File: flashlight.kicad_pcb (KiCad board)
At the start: 2 copper layers, 45 x 120 mm, 23 parts, among them J1 USB_B_Micro, J2 Conn_01x03_Pin, Q2 HSS2333, SW1 SW_DIP_x01, U1 XB4908A, U2 MT3608, U3 TP4057, U4 R6BHC-A05_LED-19-223

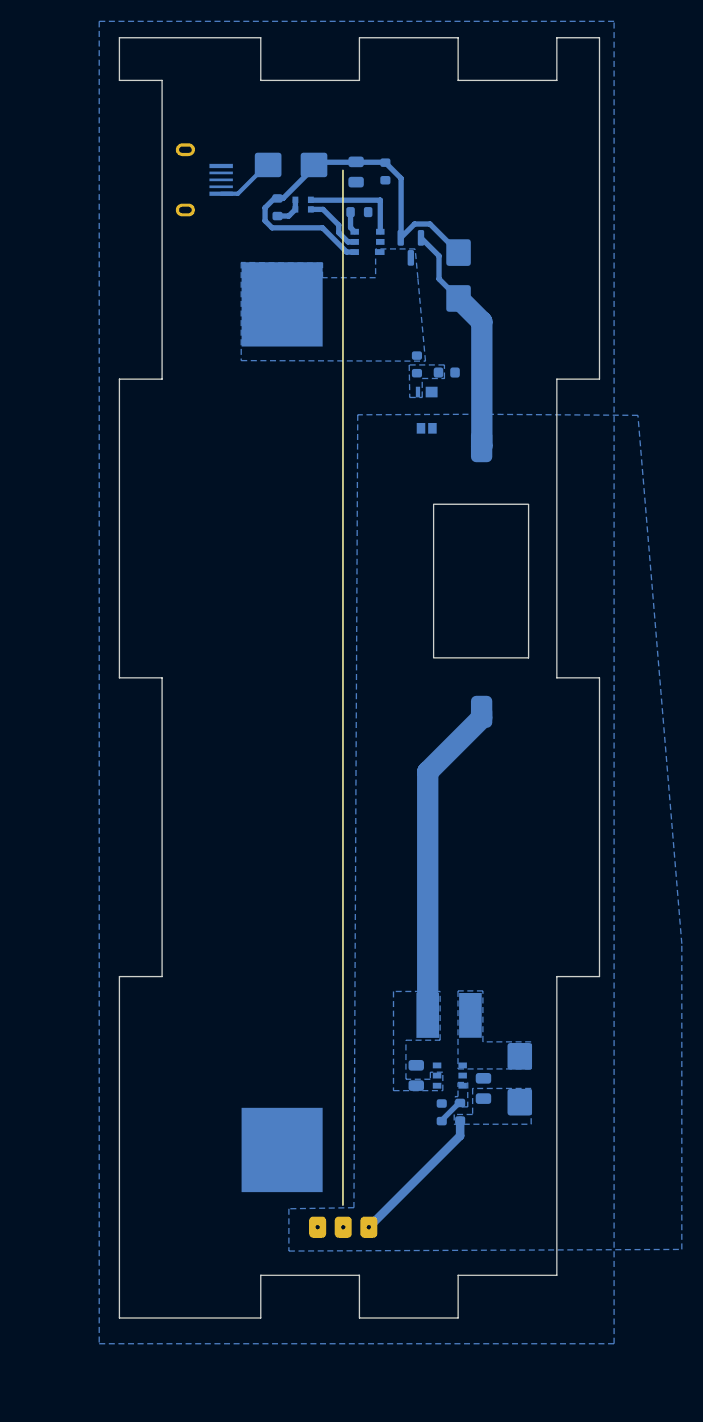
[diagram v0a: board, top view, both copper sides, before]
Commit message: v2.7 boxes
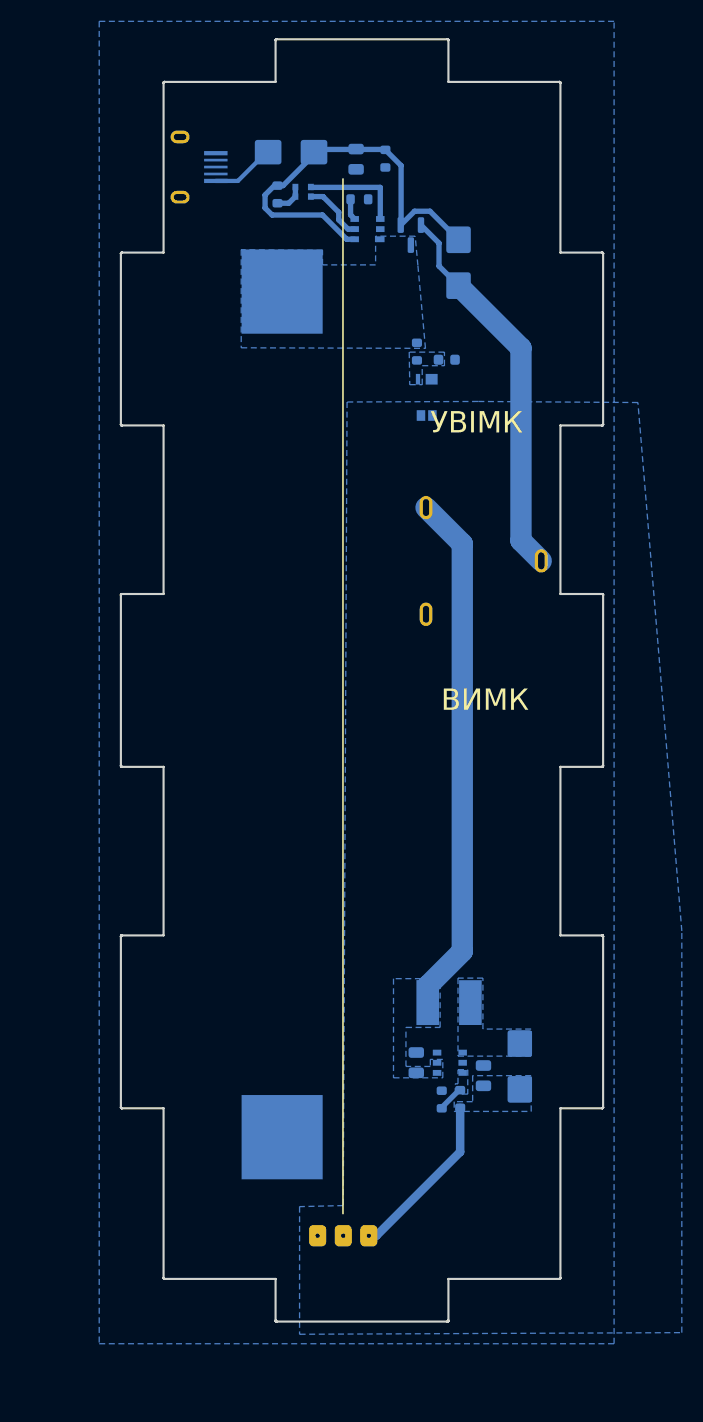
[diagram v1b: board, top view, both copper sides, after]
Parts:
- removed SW1: SW_DIP_x01, FlashlightLib:KCD11-2P
- added U5: SS12J01_071, JLCPCB-SS12J01:SW-TH_SHOU-HAN_SS12J01, F.Cu at (109.2, 84.6)
- moved J1 1.30 mm to (82.5, 47.7)
- moved C3 1.20 mm to (102.9, 131.6)
- moved C4 1.20 mm to (109.2, 132.9)
- moved R6 1.20 mm to (105.3, 135.1)
- moved U2 1.20 mm to (106.0, 131.7)
- moved BT1 1.20 mm to (90.3, 99.0)
- moved C1 1.20 mm to (97.2, 47.0)
- moved C2 1.20 mm to (105.7, 65.8)
- moved Q2 1.20 mm to (102.4, 54.1)
- moved R1 1.20 mm to (97.5, 50.7)
- moved R2 1.20 mm to (89.9, 50.3)
- moved R3 1.20 mm to (102.9, 65.0)
- moved U1 1.20 mm to (103.1, 67.6)
- moved U4 1.20 mm to (93.0, 49.5)
- moved D1 1.20 mm to (91.1, 46.3)
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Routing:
- net Net-(U2-EN): track 30.5 -> 49.1 mm
- net Net-(D4-K): track 21.9 -> 36.2 mm
- net VOUT: track 13.5 -> 16.0 mm
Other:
- board size 45 x 120 mm -> 45.2 x 120.2 mm
- board text added: "DO NOT PRINT ON F LAYER!"
- board text added: "V2.7"
- board text added: "ВИМК"
- board text added: "УВІМК"
- board text removed: "V2.6"

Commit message: V3.0 21700 3x8 leds
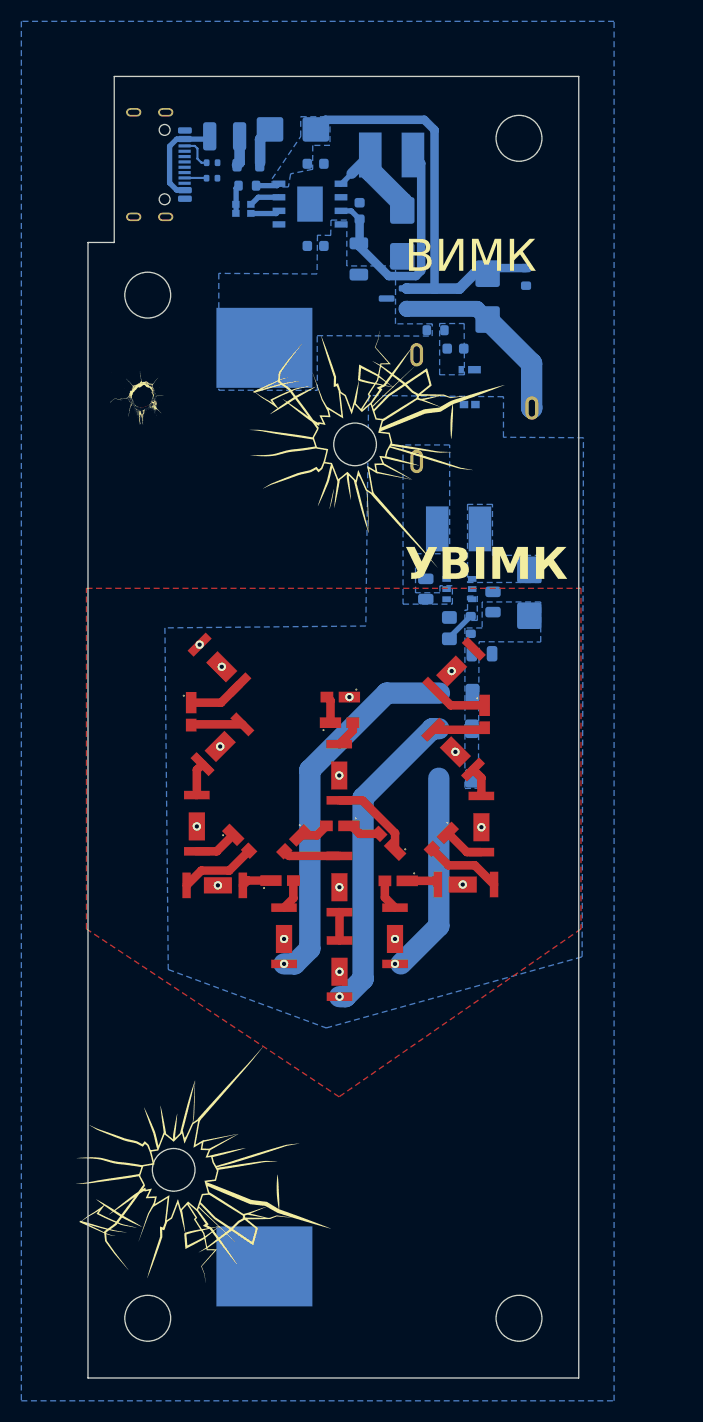
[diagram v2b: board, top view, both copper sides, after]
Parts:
- removed J1: USB_B_Micro, FlashlightLib:USB-1101IPX6-02
- removed J2: Conn_01x03_Pin, FlashlightLib:LED_Strip
- added C4: 22uF/35V, Capacitor_SMD:C_0805_2012Metric, B.Cu at (109.0, 93.3)
- added C5: 10uF/10V, Capacitor_SMD:C_0603_1608Metric, B.Cu at (97.6, 51.8)
- added C6: 10uF/10V, Capacitor_SMD:C_0603_1608Metric, B.Cu at (93.4, 55.1)
- added D10: LED, footprint:LED-SMD_L3.0-W1.4-RD_WHITE, F.Cu at (81.8, 98.9)
- added D11: LED_Pad, footprint:LED-SMD_3P-L5.7-W3.0-RD, F.Cu at (84.4, 94.3)
- added D12: LED_Pad, footprint:LED-SMD_3P-L5.7-W3.0-RD, F.Cu at (95.7, 122.8)
- added D13: LED_Pad, footprint:LED-SMD_3P-L5.7-W3.0-RD, F.Cu at (95.7, 114.9)
- added D14: LED, footprint:LED-SMD_L3.0-W1.4-RD_WHITE, F.Cu at (91.2, 111.1)
- added D15: LED, footprint:LED-SMD_L3.0-W1.4-RD_WHITE, F.Cu at (95.5, 109.4)
- added D16: LED, footprint:LED-SMD_L3.0-W1.4-RD_WHITE, F.Cu at (100.1, 110.9)
- added D17: LED_Pad, footprint:LED-SMD_3P-L5.7-W3.0-RD, F.Cu at (95.7, 104.4)
- added D18: LED, footprint:LED-SMD_L3.0-W1.4-RD_WHITE, F.Cu at (95.9, 99.8)
- added D19: LED, footprint:LED-SMD_L3.0-W1.4-RD_WHITE, F.Cu at (95.6, 97.4)
- added D2: D_Schottky, Diode_SMD:D_SMB, B.Cu at (101.6, 53.9)
- added D20: LED_Pad, footprint:LED-SMD_3P-L5.7-W3.0-RD, F.Cu at (106.4, 94.7)
- added D21: LED, footprint:LED-SMD_L3.0-W1.4-RD_WHITE, F.Cu at (109.3, 99.2)
- added D22: LED_Pad, footprint:LED-SMD_3P-L5.7-W3.0-RD, F.Cu at (106.3, 102.3)
- added D23: LED_Pad, footprint:LED-SMD_3P-L5.7-W3.0-RD, F.Cu at (109.0, 109.3)
- added D24: LED, footprint:LED-SMD_L3.0-W1.4-RD_WHITE, F.Cu at (105.1, 110.8)
- added D25: LED_Pad, footprint:LED-SMD_3P-L5.7-W3.0-RD, F.Cu at (107.5, 114.9)
- added D26: LED, footprint:LED-SMD_L3.0-W1.4-RD_WHITE, F.Cu at (101.0, 114.6)
- added D27: LED_Pad, footprint:LED-SMD_3P-L5.7-W3.0-RD, F.Cu at (100.9, 119.7)
- added D28: LED_Pad, footprint:LED-SMD_3P-L5.7-W3.0-RD, F.Cu at (90.5, 119.7)
- added D3: LED, footprint:LED-SMD_L3.0-W1.4-RD_WHITE, F.Cu at (90.3, 114.6)
- added D6: LED_Pad, footprint:LED-SMD_3P-L5.7-W3.0-RD, F.Cu at (84.0, 115.0)
- added D7: LED, footprint:LED-SMD_L3.0-W1.4-RD_WHITE, F.Cu at (86.5, 111.0)
- added D8: LED_Pad, footprint:LED-SMD_3P-L5.7-W3.0-RD, F.Cu at (82.3, 109.2)
- added D9: LED_Pad, footprint:LED-SMD_3P-L5.7-W3.0-RD, F.Cu at (84.7, 101.8)
- added F2: BSMD1210-150-6V, Fuse:Fuse_1210_3225Metric, B.Cu at (84.9, 44.8)
- added FB1: FerriteBead, Inductor_SMD:L_0805_2012Metric, B.Cu at (87.1, 47.5)
- added G***: LOGO, LOGO, F.Cu at (76.7, 69.3)
- added G***: LOGO, LOGO, F.Cu at (99.0, 74.0)
- added H1: MountingHole, FlashlightLib:M4-insert, F.Cu at (77.7, 59.7)
- added H2: MountingHole, FlashlightLib:M4-insert, F.Cu at (112.5, 45.0)
- added H3: MountingHole, FlashlightLib:M4-insert, F.Cu at (77.7, 155.6)
- added H4: MountingHole, FlashlightLib:M4-insert, F.Cu at (112.5, 155.6)
- added J11: USB_C_Receptacle_USB2.0_16P, footprint:USB-SMD_GT-USB-7070A01, B.Cu at (78.8, 47.5)
- added L2: 10uH, FlashlightLib:L_5.0x5.0, B.Cu at (100.6, 46.6)
- added R20: 5.1k, Resistor_SMD:R_0402_1005Metric, B.Cu at (83.7, 48.7)
- added R21: 5.1k, Resistor_SMD:R_0402_1005Metric, B.Cu at (83.7, 47.3)
- added R5: 33, Resistor_SMD:R_1206_3216Metric_Pad1.30x1.75mm_HandSolder, B.Cu at (106.5, 100.3)
- added R8: 0.05, Resistor_SMD:R_1206_3216Metric, B.Cu at (97.5, 56.3)
- added R9: 33, Resistor_SMD:R_1206_3216Metric_Pad1.30x1.75mm_HandSolder, B.Cu at (106.6, 97.0)
- BT1: footprint FlashlightLib:BH-18650_NoHole -> footprint:BAT-SMD_L82.5.5-W25-BH-21700-B1BJ001
- C1: value 22uF/25V -> 10uF/10V; footprint Capacitor_SMD:C_0805_2012Metric -> Capacitor_SMD:C_0603_1608Metric
- C3: value 22uF/25V -> 22uF/35V
- R1: value 1k -> 33; footprint Resistor_SMD:R_0603_1608Metric -> Resistor_SMD:R_1206_3216Metric_Pad1.30x1.75mm_HandSolder
- R6: value 10k -> 5.23k; footprint Resistor_SMD:R_0603_1608Metric -> Resistor_SMD:R_0805_2012Metric_Pad1.20x1.40mm_HandSolder
- U1: footprint FlashlightLib:XB4908A -> footprint:ESN-4_L2.8-W2.3-LS3.7-BL
- U3: value TP4057 -> TP5000; footprint SparkFun-Semiconductor-Standard:SOT23-6-Tight -> footprint:ESOP-8_L4.9-W3.9-P1.27-LS6.0-BL-EP
- U4: footprint MyFootprints:R6BHC-A05_LED -> footprint:LED-ARRAY-SMD_4P-L1.6-W1.3-BR-FD
- U5: footprint JLCPCB-SS12J01:SW-TH_SHOU-HAN_SS12J01 -> footprint:SW-TH_SHOU-HAN_SS12J01
- moved R1 55.0 mm to (106.5, 105.0)
- moved R7 44.4 mm to (108.0, 90.6)
- moved C4 44.4 mm to (110.1, 88.5)
- moved D5 44.4 mm to (113.5, 87.6)
- moved L1 44.4 mm to (106.8, 81.6)
- moved C3 44.4 mm to (103.8, 87.2)
- moved U2 44.4 mm to (106.9, 87.3)
- moved R6 44.2 mm to (106.0, 90.9)
- moved R4 17.2 mm to (113.2, 58.0)
- moved U5 14.4 mm to (108.3, 70.3)
- moved BT1 8.85 mm to (88.6, 107.7), turned to -90 degrees
- moved U4 6.63 mm to (86.7, 51.6)
- moved Q2 6.10 mm to (101.0, 60.0), turned to 180 degrees
- moved U3 5.88 mm to (92.9, 51.2), turned to -90 degrees
- moved U1 4.69 mm to (107.7, 68.3), turned to 0 degrees
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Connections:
- R1 pad 1: Net-(U3-PROG) -> Net-(D27-A)
- R1 pad 2: GND -> VOUT
- U3 pad 1: Net-(U3-~{CHRG}) -> Net-(D2-K)
- U3 pad 3: Net-(BT1-+) -> Net-(U3-VS)
- U3 pad 4: Net-(D1-K) -> Net-(BT1-+)
- U3 pad 5: Net-(U3-STDBY) -> GND
- U3 pad 6: Net-(U3-PROG) -> Net-(U3-~{STDBY})
- U4 pad 2: Net-(U3-STDBY) -> Net-(U3-~{STDBY})
- U5 pad 1: unconnected-(U5-Pad1) -> Net-(U2-EN)
- U5 pad 3: Net-(U2-EN) -> unconnected-(U5-Pad3)
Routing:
- net Net-(U2-EN): track 49.1 -> 0.00 mm
- net Net-(D28-A): track 0.00 -> 34.9 mm, vias 0 -> 1
- net Net-(D12-A): track 0.00 -> 29.7 mm, vias 0 -> 1
- net Net-(U3-VS): track 0.00 -> 23.0 mm
- net Net-(D27-A): track 0.00 -> 19.4 mm, vias 0 -> 1
- net Net-(D4-K): track 36.2 -> 18.0 mm
- net VOUT: track 16.0 -> 0.00 mm
- net Net-(D2-K): track 0.00 -> 10.5 mm
- net Net-(F2-Pad1): track 0.00 -> 9.40 mm
- net Net-(D16-K): track 0.00 -> 8.06 mm
- net Net-(D24-A): track 0.00 -> 7.22 mm
- net Net-(D6-K): track 0.00 -> 7.21 mm
- net Net-(U3-~{CHRG}): track 9.48 -> 2.83 mm
- net Net-(U3-STDBY): track 5.78 -> 0.00 mm
- net Net-(D20-A): track 0.00 -> 5.39 mm
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- added copper zone on F.Cu, net Earth_Protective
- added copper zone on B.Cu, net Net-(D1-K)
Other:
- board size 45.2 x 120.2 mm -> 46 x 122 mm
- board text added: "+"
- board text added: "V3.0"
- board text removed: "V2.7"
